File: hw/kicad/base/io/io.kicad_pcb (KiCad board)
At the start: 2 copper layers, 50 x 50 mm, 13 parts, among them J1 SPI, J10 Conn_02x20_Odd_Even, J11 ADC 2, J12 UART1, J13 Conn_02x20_Odd_Even, J2 PWM, J3 UART2, J4 I2C, J5 PWM, J6 CAN, J7 PWM, J8 PWM, J9 ADC 1

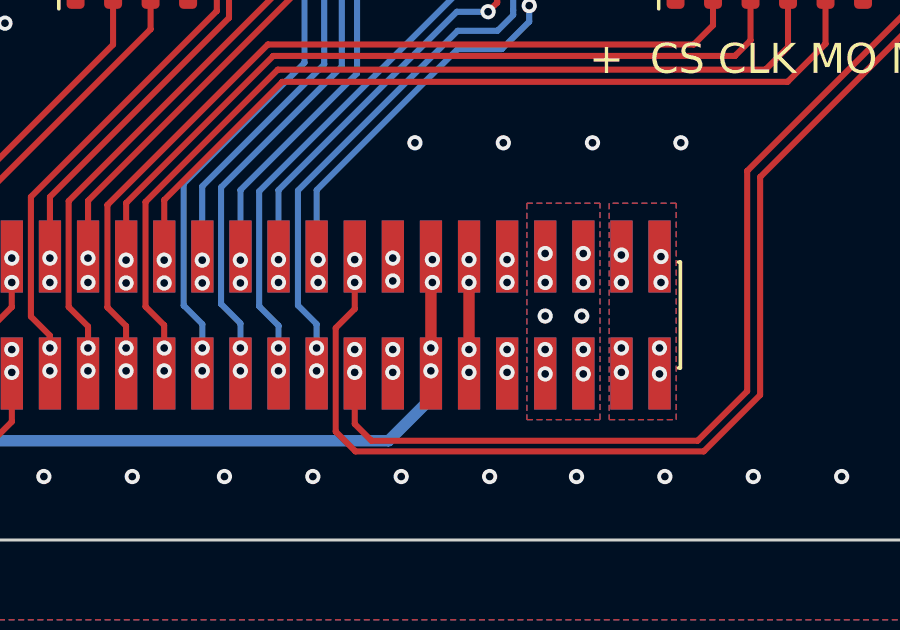
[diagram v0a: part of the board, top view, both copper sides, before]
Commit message: 更新read me
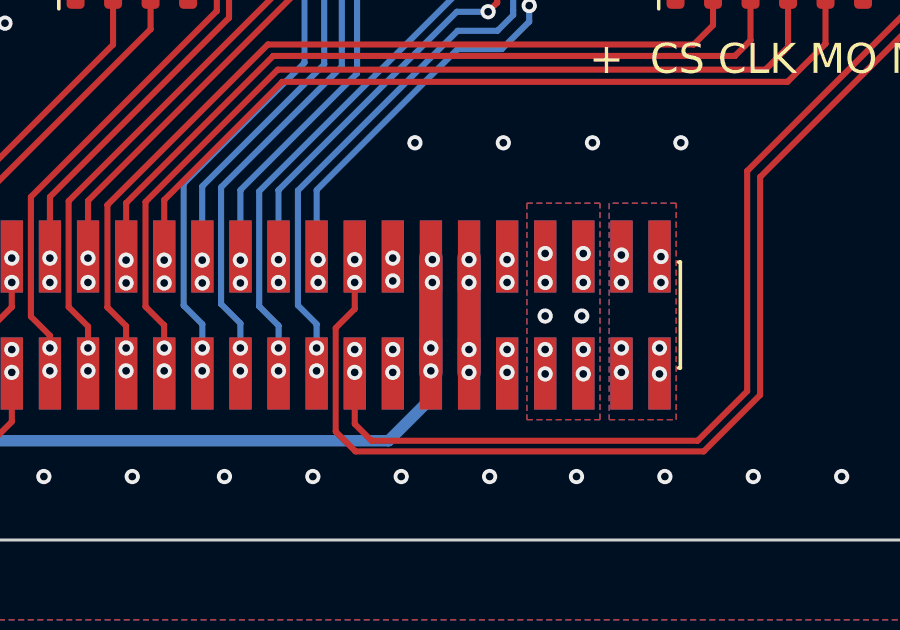
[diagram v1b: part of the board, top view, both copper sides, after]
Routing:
- net /+5V: track 3.76 -> 11.6 mm
- net +3.3V: track 205.7 -> 209.6 mm
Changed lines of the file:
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@@
   (segment (start 68.7604 40.4286) (end 79.1236 40.4286) (width 0.2032) (layer "F.Cu") (net 1))
   (segment (start 79.533532 50.4108) (end 79.533532 42.0296) (width 0.2032) (layer "F.Cu") (net 1))
-  (segment (start 80.165 71.27) (end 80.165 75.17) (width 0.381) (layer "F.Cu") (net 1))
   (segment (start 90.7852 57.4944) (end 88.293 59.9866) (width 0.2032) (layer "F.Cu") (net 1))
   (segment (start 68.293466 40.895534) (end 68.7604 40.4286) (width 0.2032) (layer "F.Cu") (net 1))
@@
   (segment (start 68.319266 52.068) (end 68.281866 52.0306) (width 0.2032) (layer "F.Cu") (net 1))
   (segment (start 79.540132 42.023) (end 79.540132 41.028068) (width 0.2032) (layer "F.Cu") (net 1))
+  (segment (start 80.165 71.27) (end 80.165 75.17) (width 0.762) (layer "F.Cu") (net 1))
   (segment (start 90.8076 52.0082) (end 90.7852 52.0306) (width 0.2032) (layer "F.Cu") (net 1))
   (segment (start 68.281866 52.0306) (end 68.281866 50.508334) (width 0.2032) (layer "F.Cu") (net 1))
@@
   (segment (start 57.051 74.49) (end 59.972 77.411) (width 0.381) (layer "B.Cu") (net 1))
   (segment (start 79.457332 50.487) (end 79.533532 50.4108) (width 0.2032) (layer "B.Cu") (net 1))
+  (segment (start 80.165 71.27) (end 80.165 75.17) (width 0.762) (layer "B.Cu") (net 1))
   (via (at 77.0662 43.7814) (size 0.508) (drill 0.254) (layers "F.Cu" "B.Cu") (net 2))
   (via (at 74.831 55.567) (size 0.508) (drill 0.254) (layers "F.Cu" "B.Cu") (net 2))
@@
   (via (at 78.8924 75.1332) (size 0.508) (drill 0.254) (layers "F.Cu" "B.Cu") (net 27))
   (via (at 78.8924 74.3712) (size 0.508) (drill 0.254) (layers "F.Cu" "B.Cu") (net 27))
+  (segment (start 81.435 71.27) (end 81.435 75.17) (width 0.762) (layer "F.Cu") (net 28))
   (segment (start 81.4324 71.374) (end 81.4324 75.1332) (width 0.381) (layer "F.Cu") (net 28))
   (via (at 81.4324 75.1332) (size 0.508) (drill 0.254) (layers "F.Cu" "B.Cu") (net 28))
@@
   (via (at 81.4324 71.374) (size 0.508) (drill 0.254) (layers "F.Cu" "B.Cu") (net 28))
   (via (at 81.4324 72.136) (size 0.508) (drill 0.254) (layers "F.Cu" "B.Cu") (net 28))
+  (segment (start 81.435 71.27) (end 81.435 75.17) (width 0.762) (layer "B.Cu") (net 28))
   (via (at 85.1916 73.2536) (size 0.508) (drill 0.254) (layers "F.Cu" "B.Cu") (free) (net 29))
   (via (at 83.9724 75.184) (size 0.508) (drill 0.254) (layers "F.Cu" "B.Cu") (net 29))
